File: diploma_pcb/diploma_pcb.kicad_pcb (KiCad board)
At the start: 2 copper layers, 50 x 24 mm, 21 parts, among them Q1 2SC3356, Q3 2SC3356

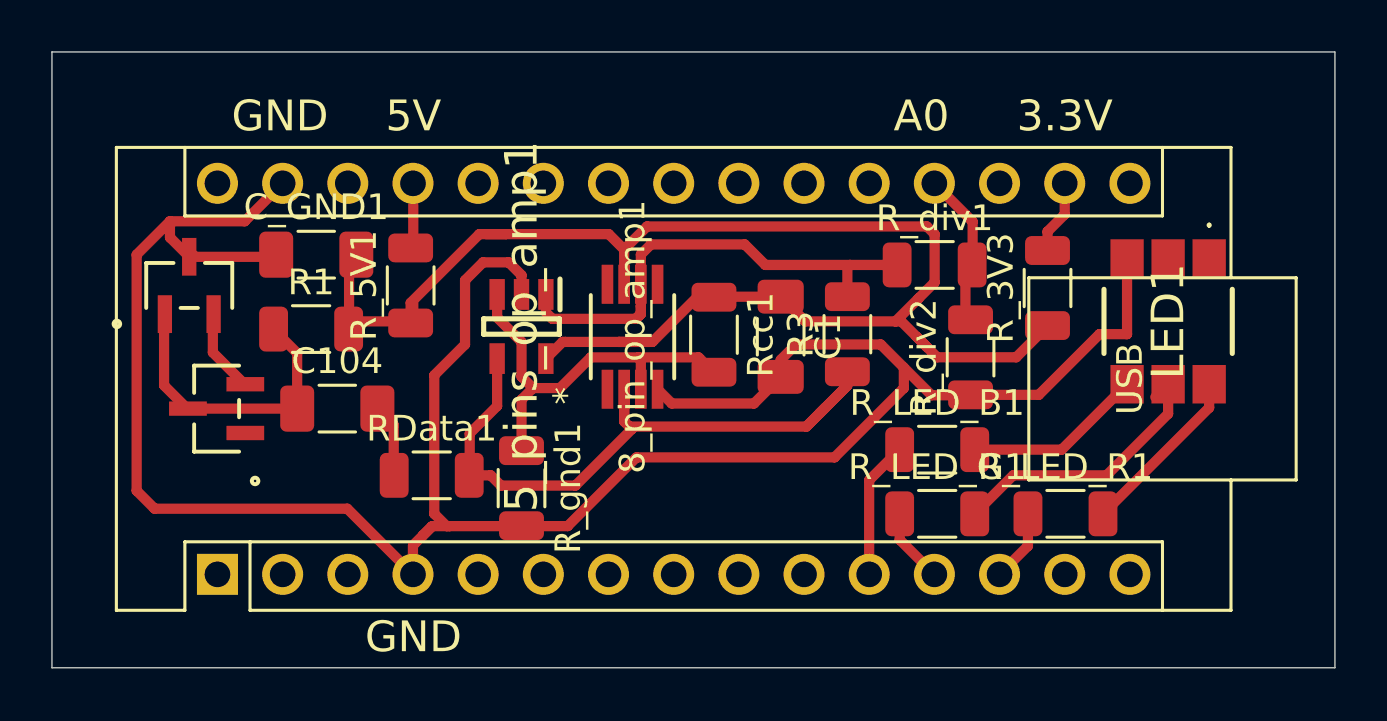
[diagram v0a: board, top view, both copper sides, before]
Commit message: fixed PCB/Word
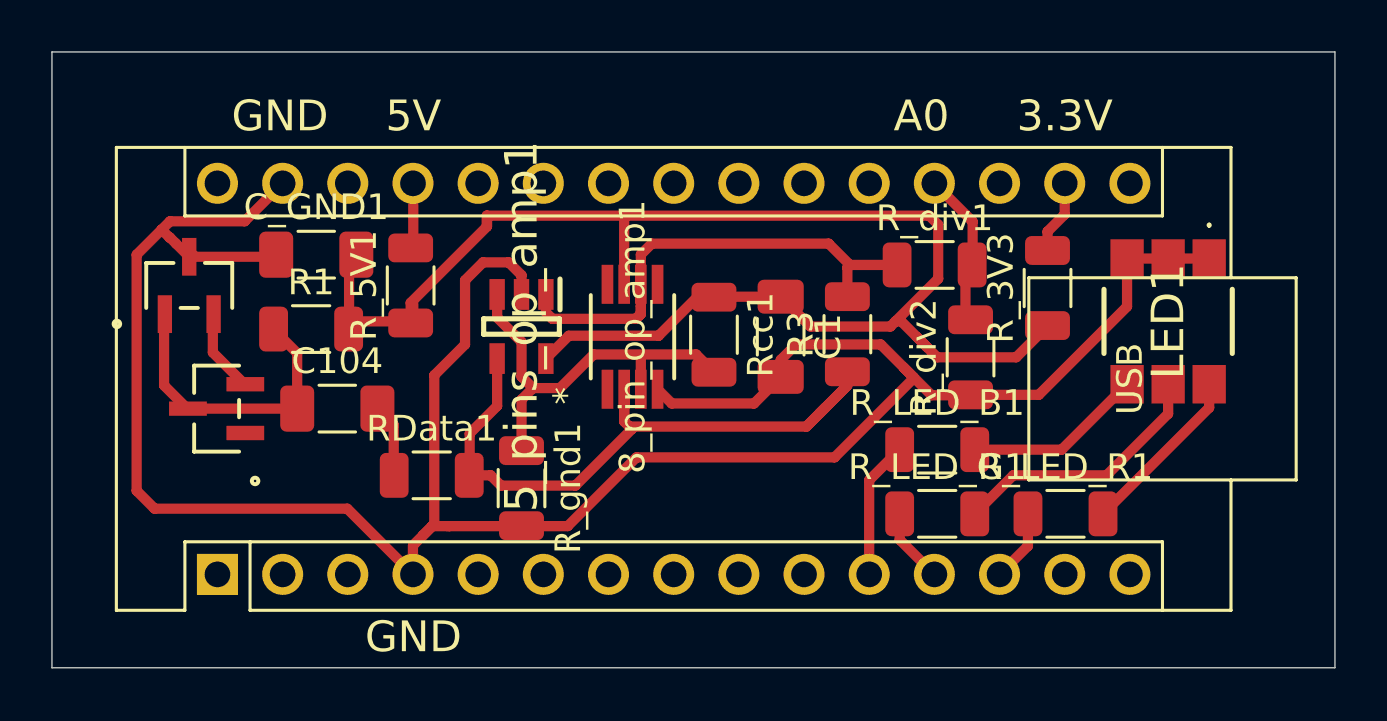
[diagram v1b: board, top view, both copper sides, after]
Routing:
- net GND: track 96.1 -> 98.6 mm
- net green: track 11.0 -> 10.3 mm
